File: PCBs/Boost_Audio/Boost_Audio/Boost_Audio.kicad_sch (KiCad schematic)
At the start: 40 parts, among them J1 XT60-M, J3 RL_Audio_From_Main, J4 To_Speaker_L, J5 To_Speaker_R, M3 CSD17581Q3, M4 CSD17581Q3A, U1 LM4752TS, U2 LM5122MH/NOPB

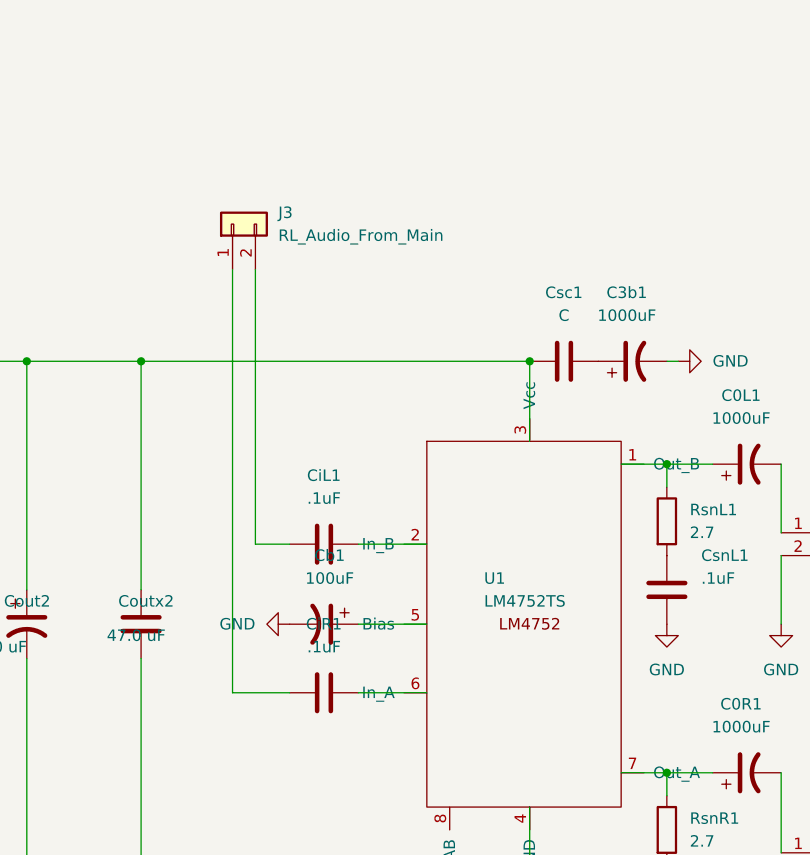
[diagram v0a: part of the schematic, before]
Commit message: new
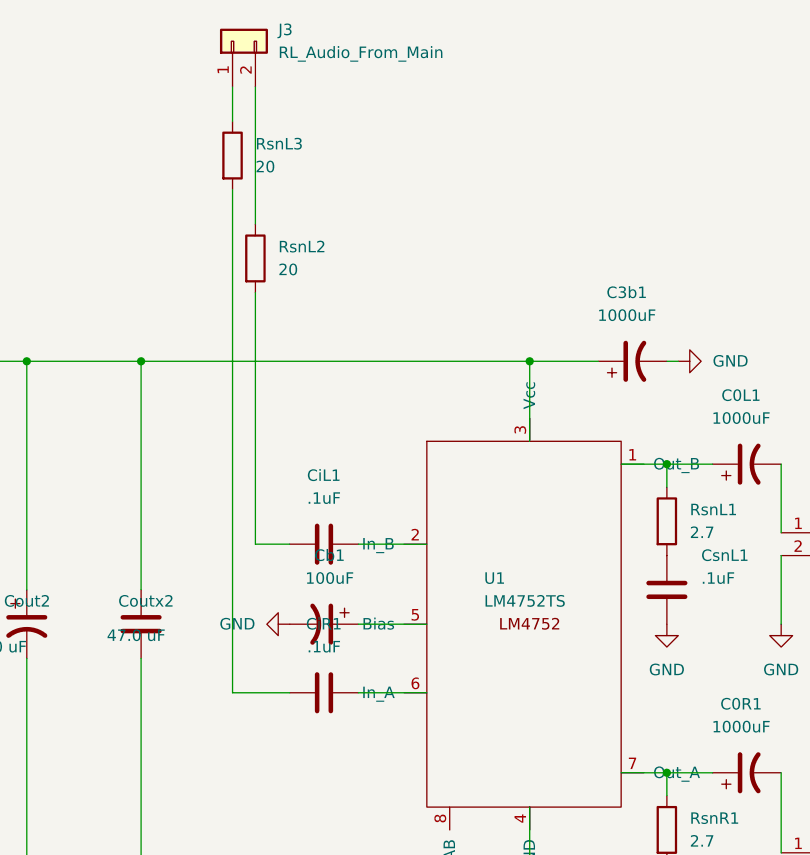
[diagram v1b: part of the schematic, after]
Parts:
- removed Csc1: C, Capacitor_SMD:C_0805_2012Metric, symbol Device:C
- added RsnL2, RsnL3: 20, Resistor_SMD:R_0805_2012Metric, symbol Device:R
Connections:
- net at Cout2.1, Coutx2.1, M4.5 (DRAIN)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: now also C3b1.1
- net at CiL1.1: now also RsnL2.2; no longer J3.2 (Pin_2)
- net at J3.1 (Pin_1): now also RsnL3.1; no longer CiR1.1
- new net: CiR1.1, RsnL3.2
- new net: J3.2 (Pin_2), RsnL2.1
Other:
- moved on the sheet: J3
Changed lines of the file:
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@@
   (junction (at 34.29 67.31) (diameter 0) (color 0 0 0 0)
   )
+  (junction (at 175.26 72.39) (diameter 0) (color 0 0 0 0)
+  )
+  (junction (at 127 132.08) (diameter 0) (color 0 0 0 0)
+  )
+  (junction (at 120.65 77.47) (diameter 0) (color 0 0 0 0)
+  )
+  (junction (at 123.19 132.08) (diameter 0) (color 0 0 0 0)
+  )
+  (junction (at 175.26 67.31) (diameter 0) (color 0 0 0 0)
+  )
+  (junction (at 203.2 67.31) (diameter 0) (color 0 0 0 0)
+  )
+  (junction (at 125.73 76.2) (diameter 0) (color 0 0 0 0)
+  )
+  (junction (at 190.5 67.31) (diameter 0) (color 0 0 0 0)
+  )
+  (junction (at 203.2 132.08) (diameter 0) (color 0 0 0 0)
+  )
+  (junction (at 147.32 99.06) (diameter 0) (color 0 0 0 0)
+  )
+  (junction (at 261.62 78.74) (diameter 0) (color 0 0 0 0)
+  )
+  (junction (at 34.29 132.08) (diameter 0) (color 0 0 0 0)
+  )
+  (junction (at 175.26 69.85) (diameter 0) (color 0 0 0 0)
+  )
   (junction (at 246.38 67.31) (diameter 0) (color 0 0 0 0)
   )
-  (junction (at 175.26 72.39) (diameter 0) (color 0 0 0 0)
-  )
-  (junction (at 127 132.08) (diameter 0) (color 0 0 0 0)
-  )
-  (junction (at 120.65 77.47) (diameter 0) (color 0 0 0 0)
-  )
-  (junction (at 123.19 132.08) (diameter 0) (color 0 0 0 0)
-  )
-  (junction (at 175.26 67.31) (diameter 0) (color 0 0 0 0)
-  )
-  (junction (at 203.2 67.31) (diameter 0) (color 0 0 0 0)
-  )
-  (junction (at 125.73 76.2) (diameter 0) (color 0 0 0 0)
-  )
-  (junction (at 190.5 67.31) (diameter 0) (color 0 0 0 0)
-  )
-  (junction (at 203.2 132.08) (diameter 0) (color 0 0 0 0)
-  )
-  (junction (at 147.32 99.06) (diameter 0) (color 0 0 0 0)
-  )
-  (junction (at 261.62 78.74) (diameter 0) (color 0 0 0 0)
-  )
-  (junction (at 34.29 132.08) (diameter 0) (color 0 0 0 0)
-  )
-  (junction (at 175.26 69.85) (diameter 0) (color 0 0 0 0)
-  )
   (junction (at 54.61 132.08) (diameter 0) (color 0 0 0 0)
   )
@@
     (stroke (width 0) (type default))
   )
+  (wire (pts (xy 246.38 67.31) (xy 254 67.31))
+    (stroke (width 0) (type default))
+  )
   (wire (pts (xy 179.07 132.08) (xy 190.5 132.08))
     (stroke (width 0) (type default))
@@
     (stroke (width 0) (type default))
   )
+  (wire (pts (xy 215.9 36.83) (xy 215.9 52.07))
+    (stroke (width 0) (type default))
+  )
   (wire (pts (xy 34.29 132.08) (xy 40.64 132.08))
     (stroke (width 0) (type default))
@@
     (stroke (width 0) (type default))
   )
+  (wire (pts (xy 213.36 36.83) (xy 213.36 40.64))
+    (stroke (width 0) (type default))
+  )
   (wire (pts (xy 110.49 95.25) (xy 128.27 95.25))
     (stroke (width 0) (type default))
@@
     (stroke (width 0) (type default))
   )
+  (wire (pts (xy 215.9 59.69) (xy 215.9 87.63))
+    (stroke (width 0) (type default))
+  )
   (wire (pts (xy 274.32 78.74) (xy 274.32 86.36))
     (stroke (width 0) (type default))
@@
     (stroke (width 0) (type default))
   )
-  (wire (pts (xy 215.9 57.15) (xy 215.9 87.63))
-    (stroke (width 0) (type default))
-  )
   (wire (pts (xy 124.46 76.2) (xy 125.73 76.2))
     (stroke (width 0) (type default))
@@
     (stroke (width 0) (type default))
   )
-  (wire (pts (xy 213.36 57.15) (xy 213.36 104.14))
-    (stroke (width 0) (type default))
-  )
   (wire (pts (xy 74.93 80.01) (xy 74.93 87.63))
     (stroke (width 0) (type default))
@@
   )
   (wire (pts (xy 130.81 91.44) (xy 139.7 91.44))
+    (stroke (width 0) (type default))
+  )
+  (wire (pts (xy 213.36 48.26) (xy 213.36 104.14))
     (stroke (width 0) (type default))
   )
@@
     )
   )
+  (symbol (lib_id "Device:R") (at 213.36 44.45 0) (unit 1)
+    (in_bom yes) (on_board yes) (dnp no) (fields_autoplaced)
+    (property "Reference" "RsnL3" (at 215.9 43.18 0)
+      (effects (font (size 1.27 1.27)) (justify left))
+    )
+    (property "Value" "20" (at 215.9 45.72 0)
+      (effects (font (size 1.27 1.27)) (justify left))
+    )
+    (property "Footprint" "Resistor_SMD:R_0805_2012Metric" (at 211.582 44.45 90)
+      (effects (font (size 1.27 1.27)) hide)
+    )
+    (property "Datasheet" "~" (at 213.36 44.45 0)
+      (effects (font (size 1.27 1.27)) hide)
+    )
+    (pin "1")
+    (pin "2")
+    (instances
+      (project "Boost_Audio"
+        (path "/fd5b3421-9c2a-40d1-9fed-b28030b8ba38"
+          (reference "RsnL3") (unit 1)
+        )
+      )
+    )
+  )
   (symbol (lib_id "power:GND") (at 274.32 96.52 0) (unit 1)
     (in_bom yes) (on_board yes) (dnp no) (fields_autoplaced)
@@
         (path "/fd5b3421-9c2a-40d1-9fed-b28030b8ba38"
           (reference "Cvcc2") (unit 1)
-        )
-      )
-    )
-  )
-  (symbol (lib_id "Device:C") (at 250.19 67.31 90) (unit 1)
-    (in_bom yes) (on_board yes) (dnp no) (fields_autoplaced)
-    (property "Reference" "Csc1" (at 250.19 59.69 90)
-      (effects (font (size 1.27 1.27)))
-    )
-    (property "Value" "C" (at 250.19 62.23 90)
-      (effects (font (size 1.27 1.27)))
-    )
-    (property "Footprint" "Capacitor_SMD:C_0805_2012Metric" (at 254 66.3448 0)
-      (effects (font (size 1.27 1.27)) hide)
-    )
-    (property "Datasheet" "~" (at 250.19 67.31 0)
-      (effects (font (size 1.27 1.27)) hide)
-    )
-    (pin "2")
-    (pin "1")
-    (instances
-      (project "Boost_Audio"
-        (path "/fd5b3421-9c2a-40d1-9fed-b28030b8ba38"
-          (reference "Csc1") (unit 1)
         )
       )
@@
     )
   )
-  (symbol (lib_id "Connector_Generic:Conn_01x02") (at 213.36 52.07 90) (unit 1)
-    (in_bom yes) (on_board yes) (dnp no) (fields_autoplaced)
-    (property "Reference" "J3" (at 218.44 50.8 90)
+  (symbol (lib_id "Device:R") (at 215.9 55.88 0) (unit 1)
+    (in_bom yes) (on_board yes) (dnp no) (fields_autoplaced)
+    (property "Reference" "RsnL2" (at 218.44 54.61 0)
+      (effects (font (size 1.27 1.27)) (justify left))
+    )
+    (property "Value" "20" (at 218.44 57.15 0)
+      (effects (font (size 1.27 1.27)) (justify left))
+    )
+    (property "Footprint" "Resistor_SMD:R_0805_2012Metric" (at 214.122 55.88 90)
+      (effects (font (size 1.27 1.27)) hide)
+    )
+    (property "Datasheet" "~" (at 215.9 55.88 0)
+      (effects (font (size 1.27 1.27)) hide)
+    )
+    (pin "1")
+    (pin "2")
+    (instances
+      (project "Boost_Audio"
+        (path "/fd5b3421-9c2a-40d1-9fed-b28030b8ba38"
+          (reference "RsnL2") (unit 1)
+        )
+      )
+    )
+  )
+  (symbol (lib_id "Connector_Generic:Conn_01x02") (at 213.36 31.75 90) (unit 1)
+    (in_bom yes) (on_board yes) (dnp no) (fields_autoplaced)
+    (property "Reference" "J3" (at 218.44 30.48 90)
       (effects (font (size 1.27 1.27)) (justify right))
     )
-    (property "Value" "RL_Audio_From_Main" (at 218.44 53.34 90)
+    (property "Value" "RL_Audio_From_Main" (at 218.44 33.02 90)
       (effects (font (size 1.27 1.27)) (justify right))
     )
-    (property "Footprint" "Connector_JST:JST_EH_B2B-EH-A_1x02_P2.50mm_Vertical" (at 213.36 52.07 0)
-      (effects (font (size 1.27 1.27)) hide)
-    )
-    (property "Datasheet" "~" (at 213.36 52.07 0)
-      (effects (font (size 1.27 1.27)) hide)
-    )
+    (property "Footprint" "Connector_JST:JST_EH_B2B-EH-A_1x02_P2.50mm_Vertical" (at 213.36 31.75 0)
+      (effects (font (size 1.27 1.27)) hide)
+    )
+    (property "Datasheet" "~" (at 213.36 31.75 0)
+      (effects (font (size 1.27 1.27)) hide)
+    )
